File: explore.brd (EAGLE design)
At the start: 68.6 x 55.9 mm, 11 parts

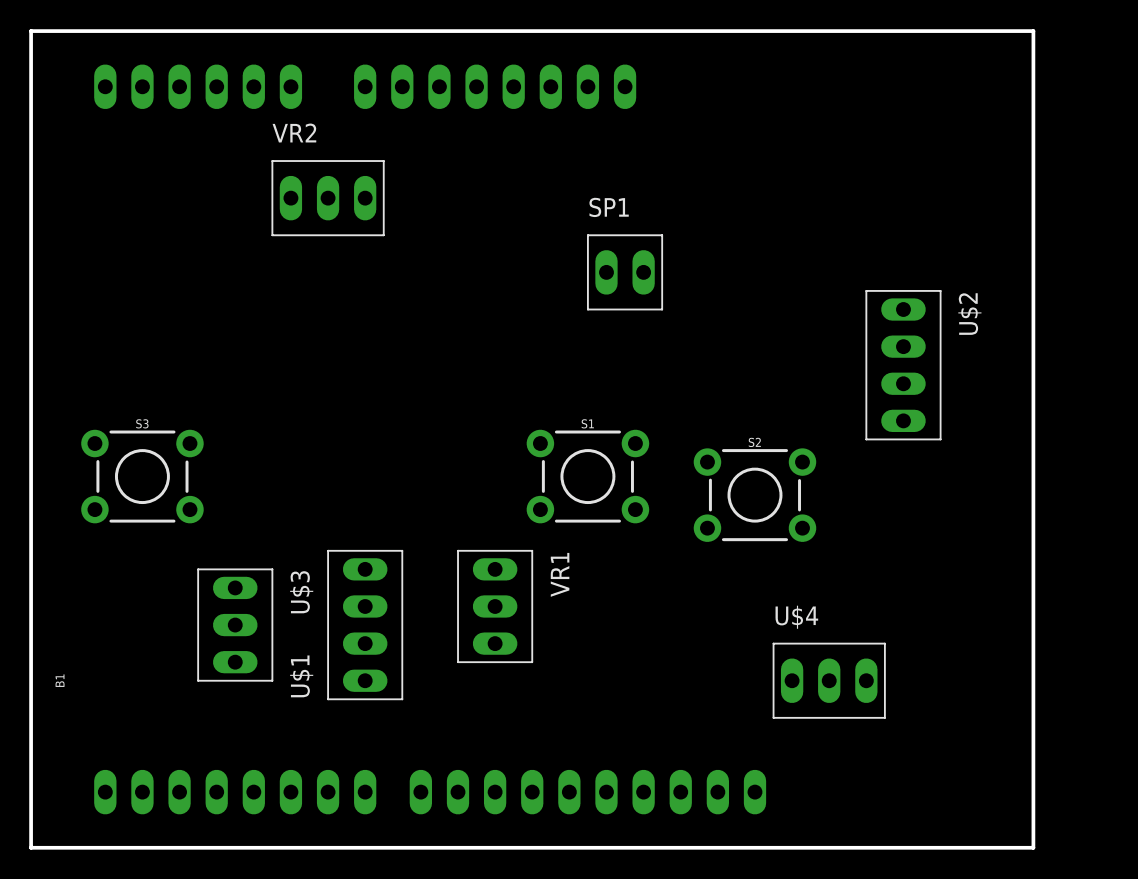
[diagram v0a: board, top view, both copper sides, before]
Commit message: finihed and checked first draft
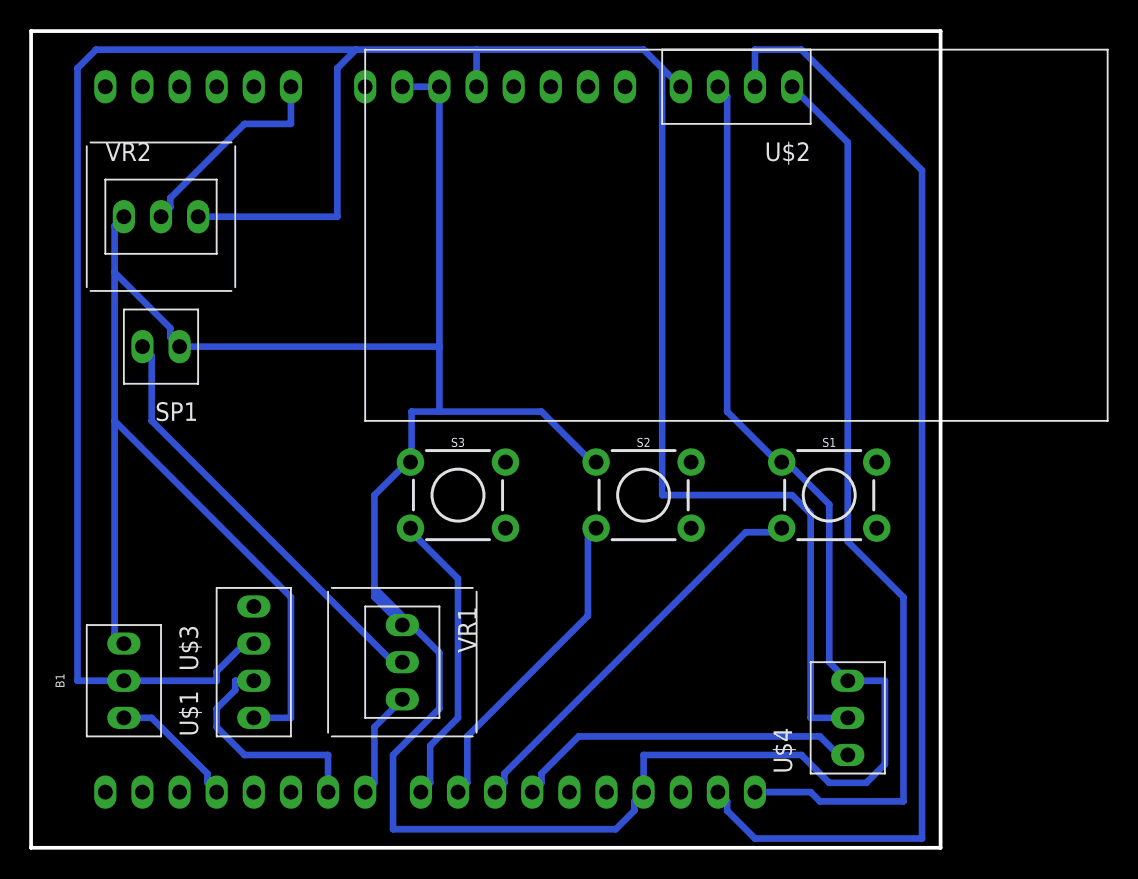
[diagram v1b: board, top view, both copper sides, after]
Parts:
- U$2: value 4DIGITDISPLAY -> 4DIGITDISPLAYOUTLINE; device christy:4-HOLE-LARGE -> christy:4DIGITDISPLAY
- VR1, VR2: device christy:3-HOLE-LARGE -> christy:POTENTIOMETER
- moved SP1 32.2 mm to (8.89, 33.0), turned to 180 degrees
- moved U$2 22.2 mm to (48.3, 50.8), turned to 180 degrees
- moved S3 21.6 mm to (29.2, 22.9)
- moved S1 16.6 mm to (54.6, 22.9)
- moved VR2 11.5 mm to (8.89, 41.9)
- moved U$3 8.52 mm to (6.35, 10.2)
- moved U$1 8.03 mm to (15.2, 11.4)
- moved S2 7.62 mm to (41.9, 22.9)
- moved VR1 7.41 mm to (25.4, 11.4)
- moved U$4 2.84 mm to (55.9, 7.62), turned to 90 degrees
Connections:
- net +5V: now also U$2.4; no longer U$2.P$1
- net BTN1: now also B1.D10
- net BTN2: now also B1.D9
- net BTN3: now also B1.D8
- net GND: now also U$2.3; no longer U$2.P$2
- net SCL: now also U$2.1; no longer U$2.P$4
- net SDA: now also U$2.2; no longer U$2.P$3
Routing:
- net GND: track 0.00 -> 249.4 mm
- net +5V: track 0.00 -> 178.7 mm
- net SDA: track 0.00 -> 78.8 mm
- net SCL: track 0.00 -> 62.5 mm
- net N$2: track 0.00 -> 29.3 mm
- net BTN1: track 0.00 -> 27.4 mm
- net IRC: track 0.00 -> 24.1 mm
- net BTN2: track 0.00 -> 22.1 mm
- net BTN3: track 0.00 -> 20.4 mm
- net DIN: track 0.00 -> 15.9 mm
- net N$1: track 0.00 -> 14.4 mm
- net SIG: track 0.00 -> 8.83 mm
- net PZO: track 0.00 -> 7.40 mm
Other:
- board size 68.6 x 55.9 mm -> 62.2 x 55.9 mm
